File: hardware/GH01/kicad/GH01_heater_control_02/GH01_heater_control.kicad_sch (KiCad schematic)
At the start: 9 parts, among them Q1 Q_NMOS_GDS, U1 XIAO ESP32C3, U2 CX240D5

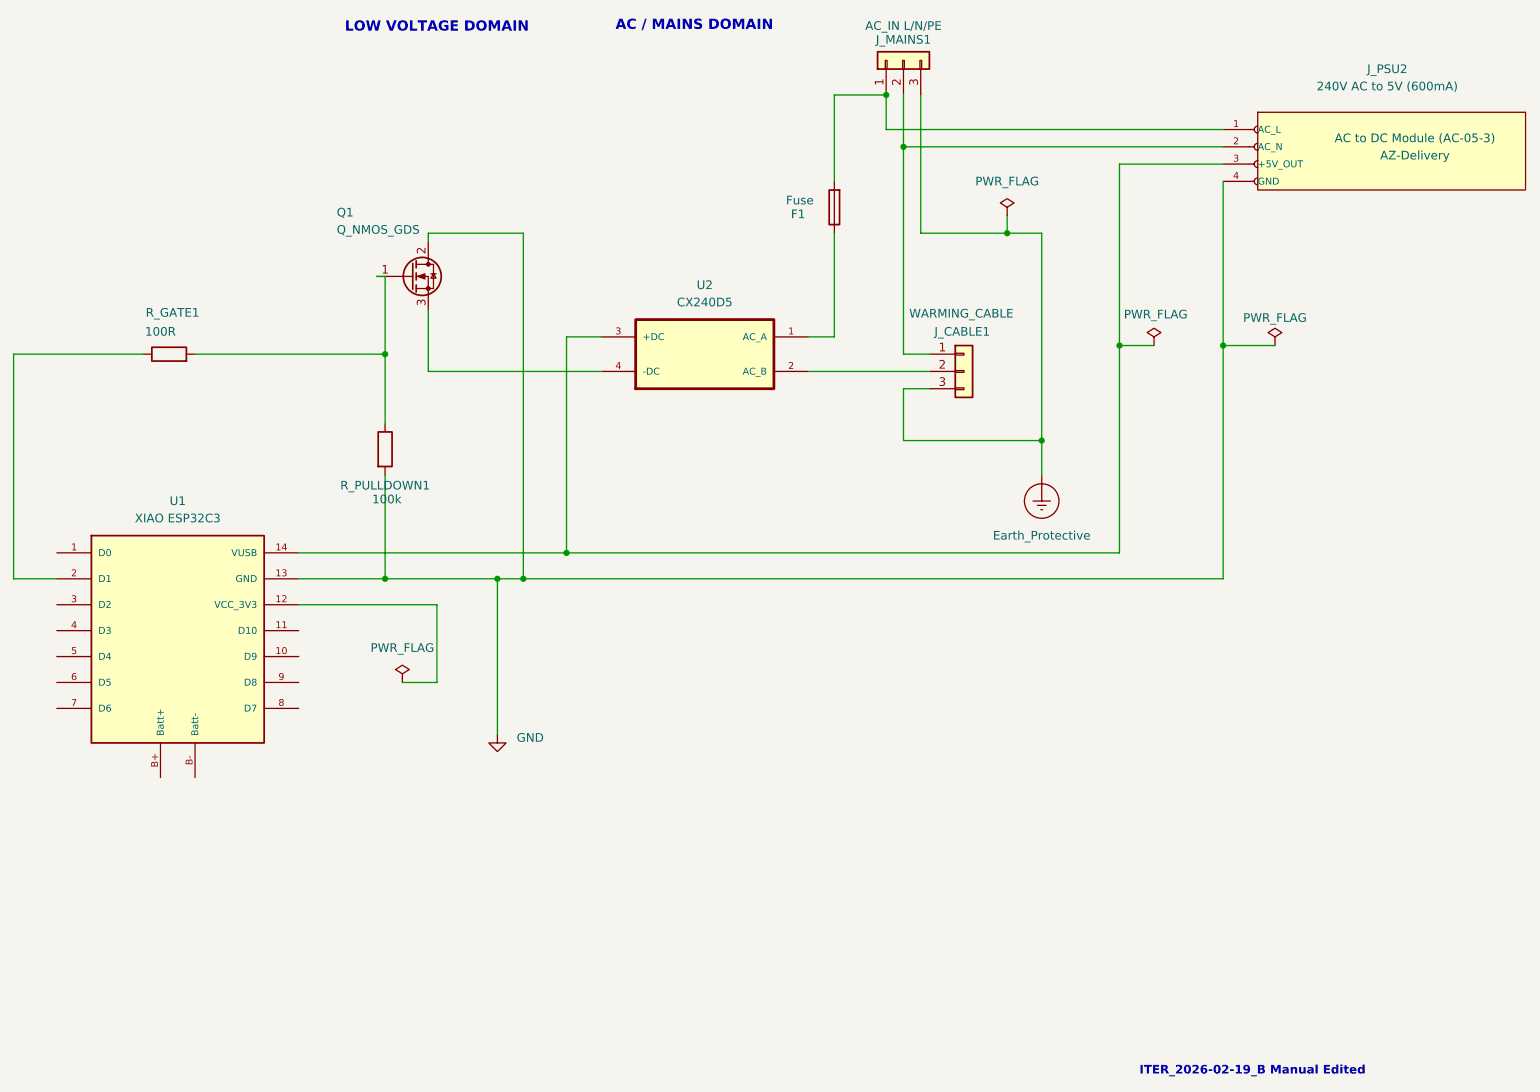
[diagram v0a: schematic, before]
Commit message: GH01 V2 design updates
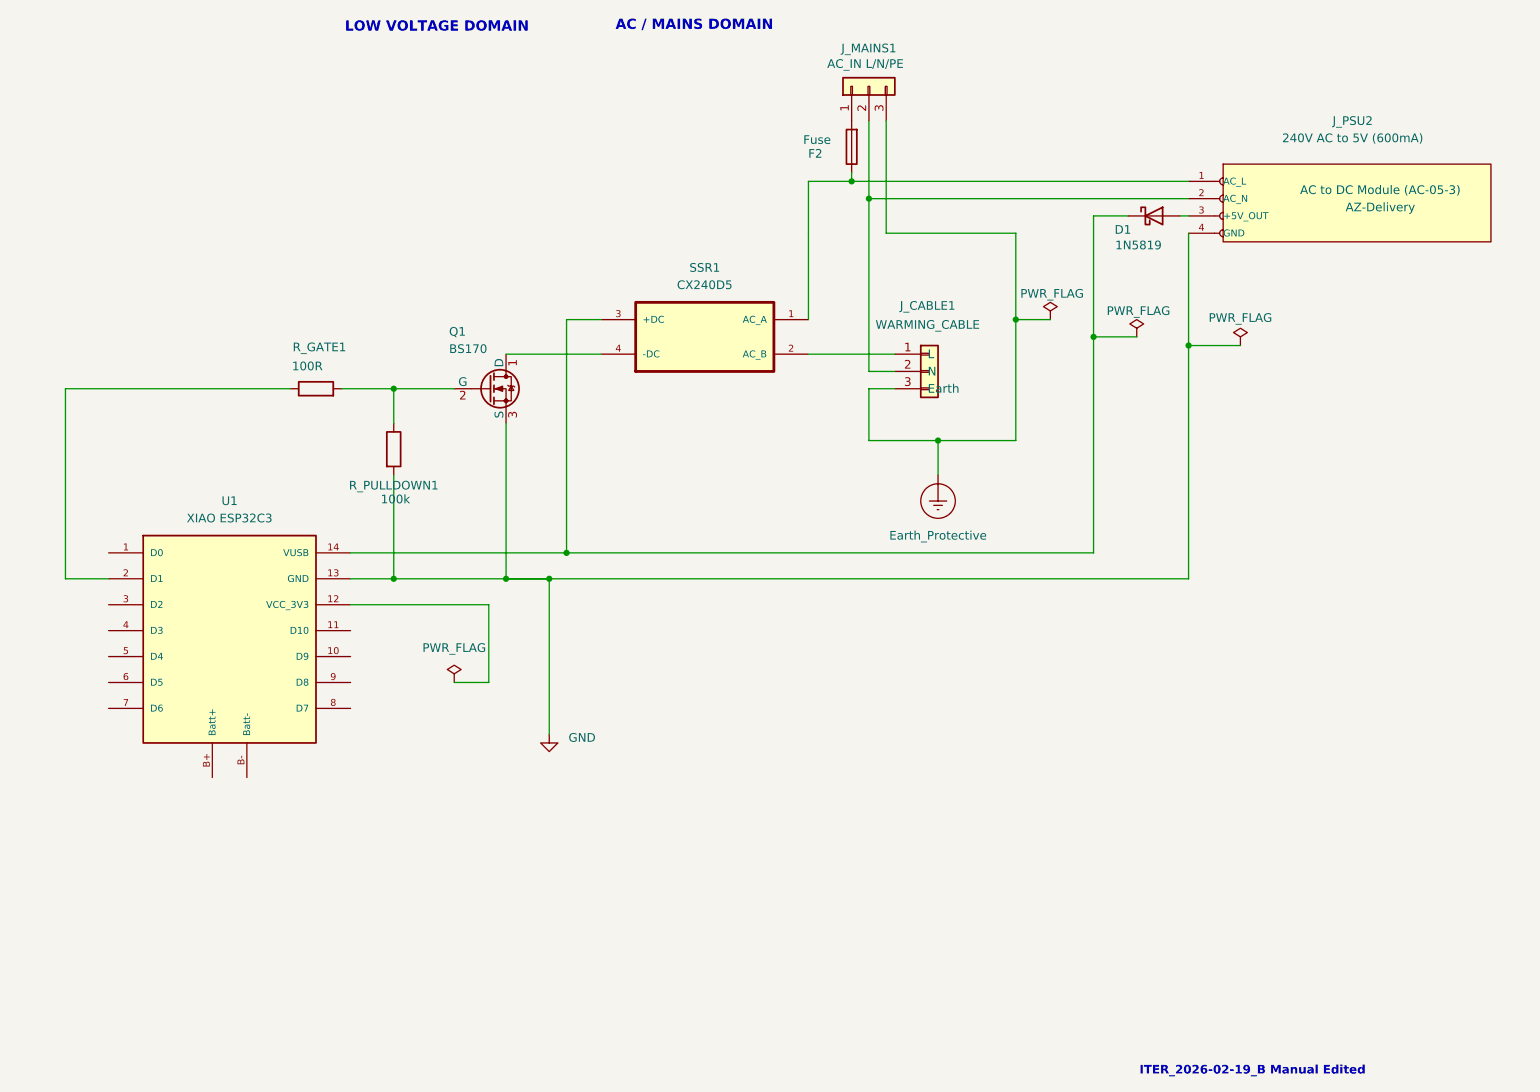
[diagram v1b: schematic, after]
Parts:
- removed F1: Fuse, symbol Device:Fuse
- removed Q1: Q_NMOS_GDS, symbol Transistor_FET:Q_NMOS_GDS
- added D1: 1N5819, Diode_THT:D_DO-41_SOD81_P10.16mm_Horizontal, symbol Diode:1N5819
- added F2: Fuse, symbol Device:Fuse
- added Q1: BS170, Package_TO_SOT_THT:TO-92_Inline, symbol Transistor_FET:BS170
- renumbered U2 to SSR1
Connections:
- net GND: now also Q1.3 (S)
- net at SSR1.1 (AC_A): now also J_PSU2.1 (AC_L), F2.1
- net at J_MAINS1.1 (Pin_1): now also F2.2; no longer J_PSU2.1 (AC_L)
- net at SSR1.2 (AC_B): now also J_CABLE1.1 (L); no longer J_CABLE1.2 (Pin_2)
- net at SSR1.3 (+DC), U1.14 (VUSB): now also D1.1 (K); no longer J_PSU2.3 (+5V_OUT)
- net at SSR1.4 (-DC): now also Q1.1 (D)
- net at J_MAINS1.2 (Pin_2), J_PSU2.2 (AC_N): now also J_CABLE1.2 (N); no longer J_CABLE1.1 (Pin_1)
- net at R_GATE1.2, R_PULLDOWN1.1: now also Q1.2 (G)
- new net: D1.2 (A), J_PSU2.3 (+5V_OUT)
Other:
- moved on the sheet: J_MAINS1, J_PSU2, R_GATE1, R_PULLDOWN1, SSR1, U1
